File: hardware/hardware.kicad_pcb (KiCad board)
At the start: 2 copper layers, 20 parts, among them J1 Conn_01x04_Male, J2 DIN-5_180degree, J3 DIN-5_180degree, SW1 SW_Push, U1 Teensy3.2, U2 TeensyAudioShield3.2, U3 6N139

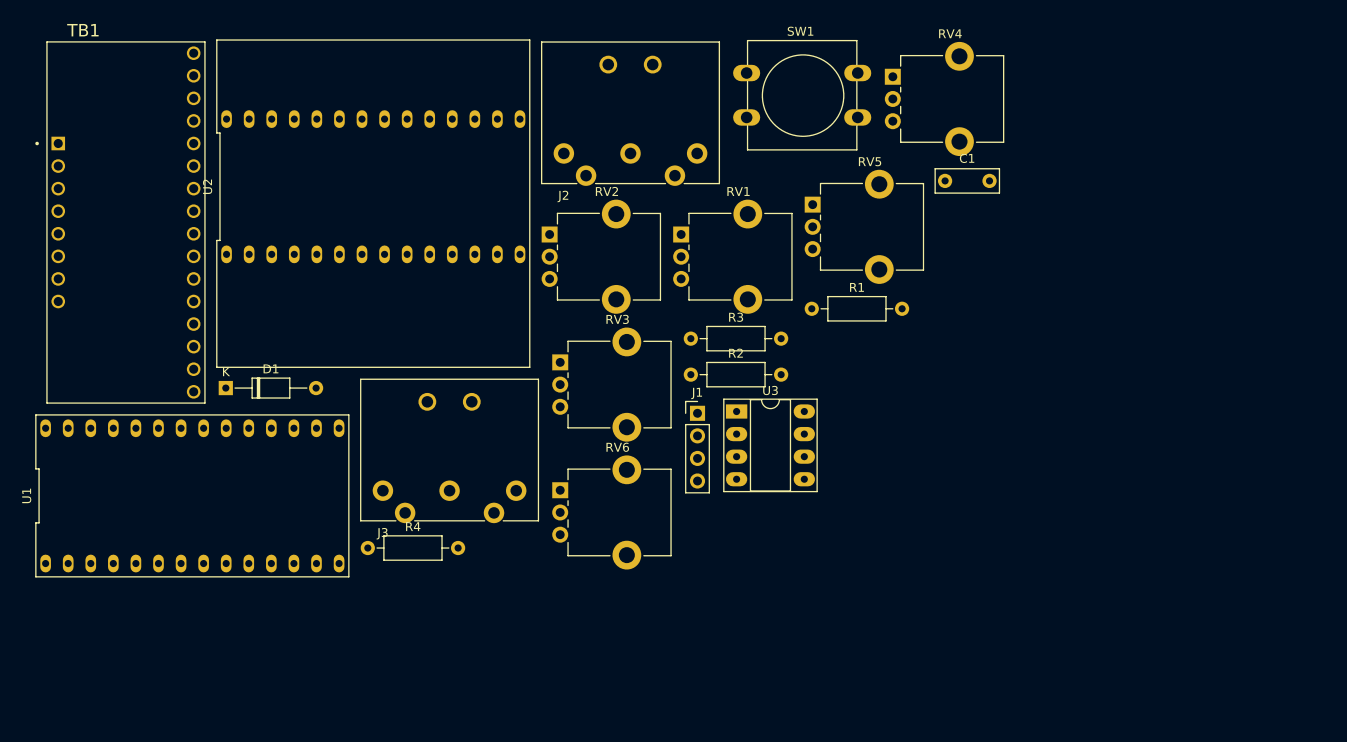
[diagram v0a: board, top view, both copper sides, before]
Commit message: Layout pcb
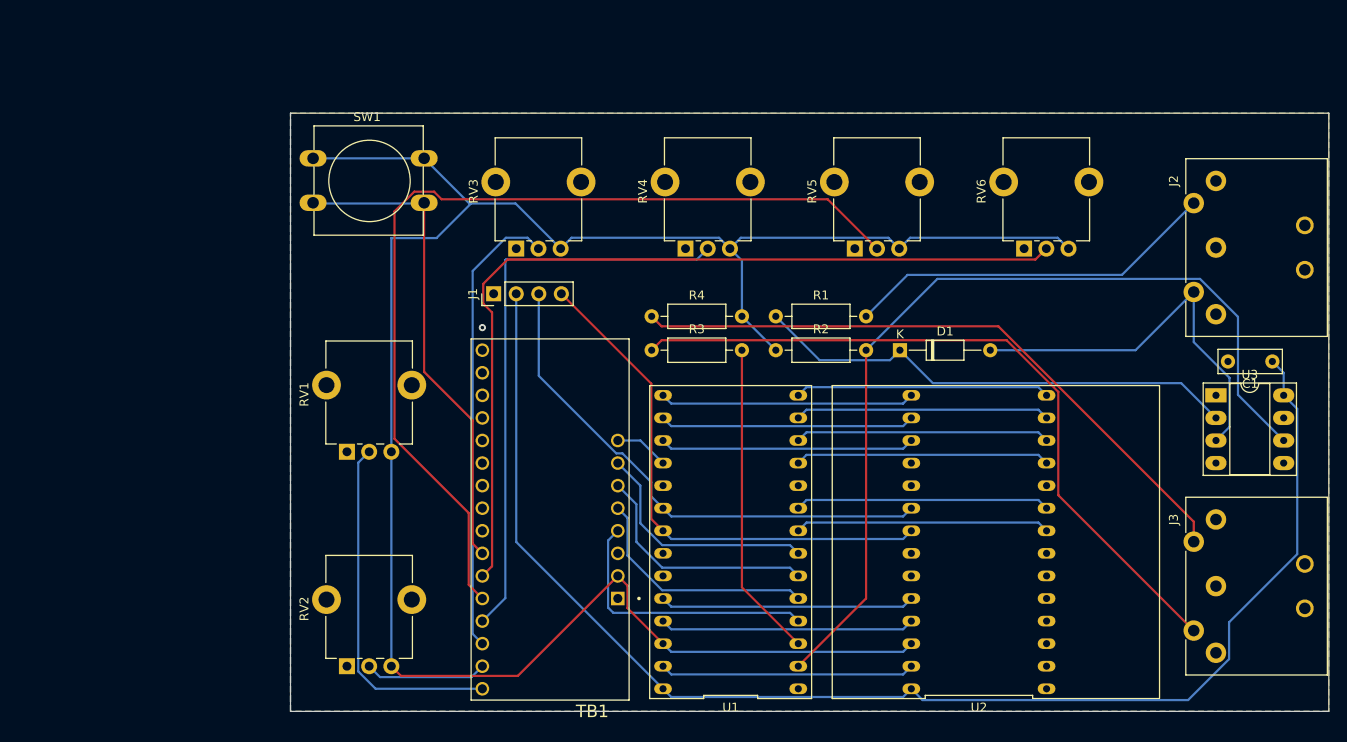
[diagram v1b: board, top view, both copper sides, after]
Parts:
- moved J3 93.8 mm to (174.0, 134.6), turned to 270 degrees
- moved U2 79.0 mm to (147.3, 137.2), turned to 90 degrees
- moved D1 76.0 mm to (138.4, 115.6)
- moved J2 73.4 mm to (174.0, 96.5), turned to 270 degrees
- moved U1 60.8 mm to (119.4, 137.2), turned to 90 degrees
- moved RV6 58.9 mm to (152.4, 104.1), turned to 90 degrees
- moved TB1 58.3 mm to (99.1, 134.6), turned to 180 degrees
- moved U3 54.0 mm to (174.0, 120.7)
- moved RV2 53.7 mm to (76.2, 151.1), turned to 90 degrees
- moved SW1 49.7 mm to (72.4, 94.0)
- moved RV1 44.9 mm to (76.2, 127.0), turned to 90 degrees
- moved C1 42.1 mm to (180.3, 116.8), turned to 180 degrees
- moved R4 41.2 mm to (110.5, 111.8)
- moved RV4 30.3 mm to (114.3, 104.1), turned to 90 degrees
- moved J1 26.6 mm to (92.7, 109.2), turned to 90 degrees
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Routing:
- net +3V3: track 0.00 -> 233.6 mm
- net +5V: track 0.00 -> 156.0 mm
- net /ADSR_Sustain: track 0.00 -> 105.5 mm
- net /MIDI_IN: track 0.00 -> 101.7 mm
- net /ADSR_Release: track 0.00 -> 98.7 mm
- net Net-(J3-Pad5): track 0.00 -> 81.8 mm
- net Net-(J3-Pad4): track 0.00 -> 72.8 mm
- net /ADSR_Decay: track 0.00 -> 65.0 mm
- net /SCL: track 0.00 -> 60.1 mm
- net /SDA: track 0.00 -> 59.0 mm
- net Net-(D1-Pad1): track 0.00 -> 55.2 mm
- net /OSC1_WAV: track 0.00 -> 54.7 mm
- net /ADSR_Attack: track 0.00 -> 51.8 mm
- net Net-(D1-Pad2): track 0.00 -> 44.6 mm
- net Net-(J2-Pad4): track 0.00 -> 42.1 mm
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- added copper zone on B.Cu, net GND
- added copper zone on F.Cu, net GND
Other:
- board outline added: 116.8 x 67.3 mm
